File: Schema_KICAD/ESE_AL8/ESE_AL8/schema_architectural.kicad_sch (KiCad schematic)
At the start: 0 parts

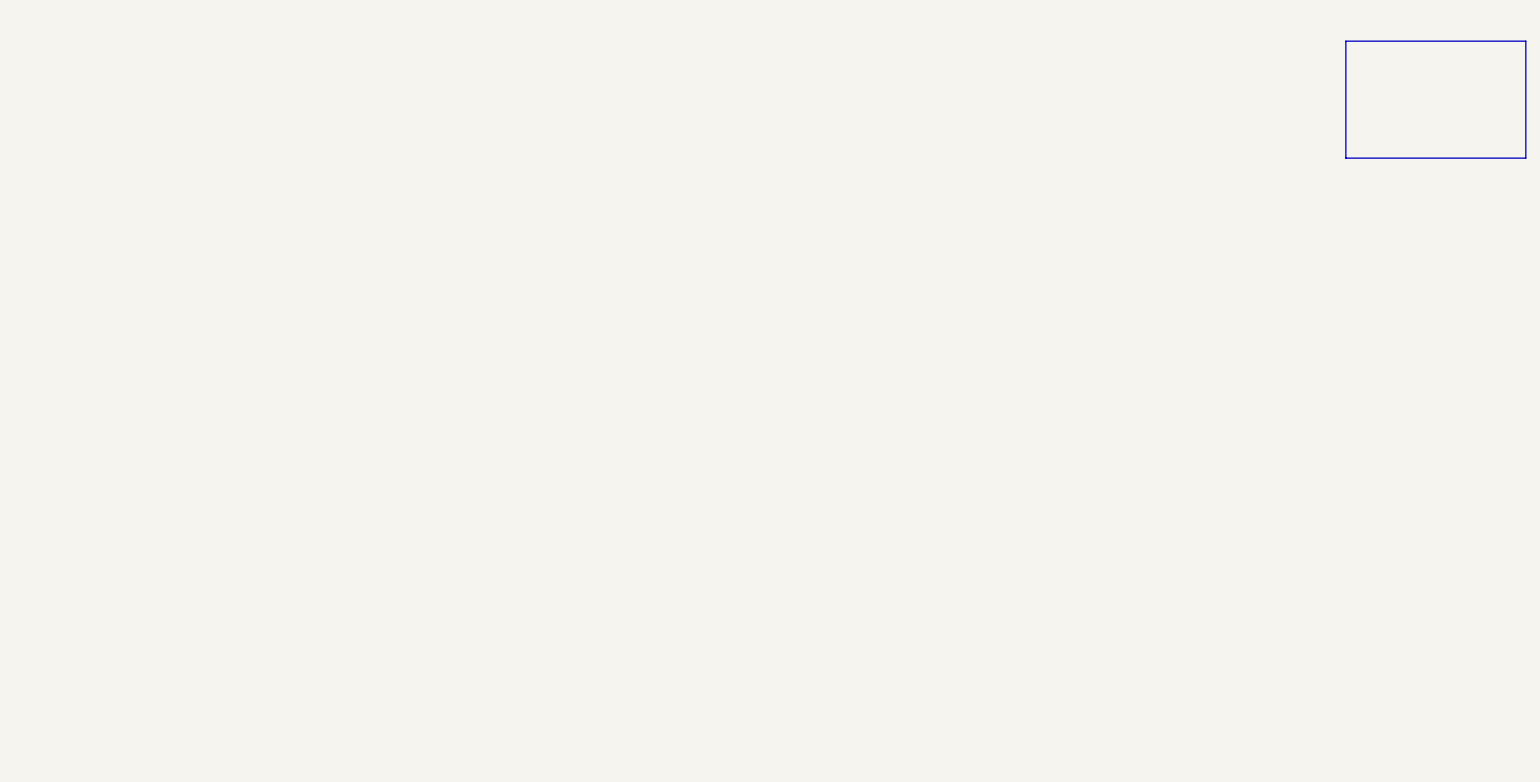
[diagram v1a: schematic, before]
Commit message: schema
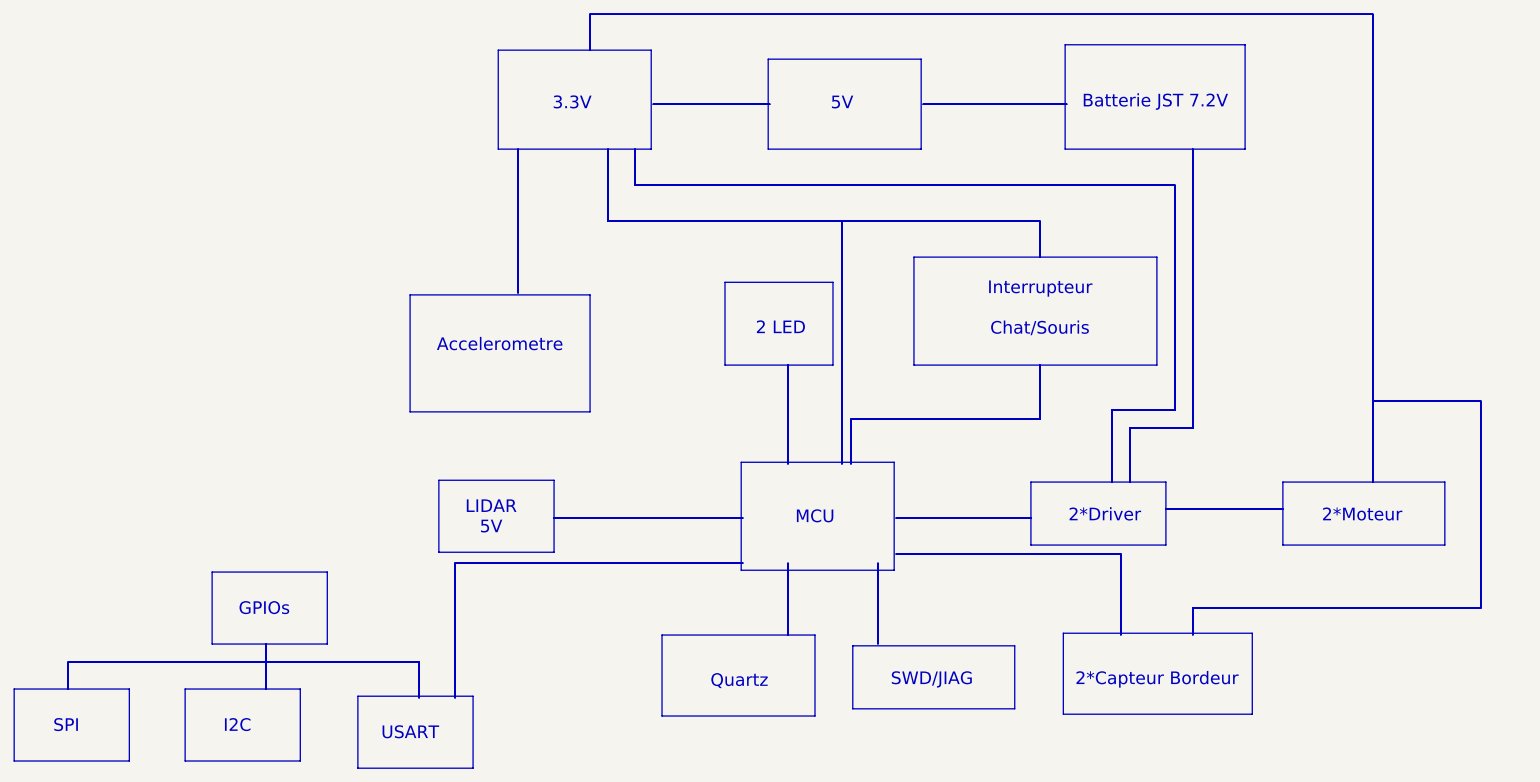
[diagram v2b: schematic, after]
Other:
- note added: "2 LED"
- note added: "2*Capteur Bordeur"
- note added: "2*Driver"
- note added: "2*Moteur"
- note added: "3.3V"
- note added: "5V"
- note added: "Accelerometre"
- note added: "Batterie JST 7.2V"
- note added: "GPIOs"
- note added: "I2C"
- note added: "Interrupteur Chat/Souris"
- note added: "LIDAR 5V"
- note added: "MCU"
- note added: "Quartz"
- note added: "SPI"
- note added: "SWD/JIAG"
- note added: "USART"
